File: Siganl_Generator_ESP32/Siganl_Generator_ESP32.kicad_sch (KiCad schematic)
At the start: 25 parts, among them J1 Conn_01x04_Socket, J2 Conn_01x02_Socket, J4 Conn_01x19_Socket, SW1 SW_Push, SW2 SW_Push, SW3 SW_Push, U2 LM393

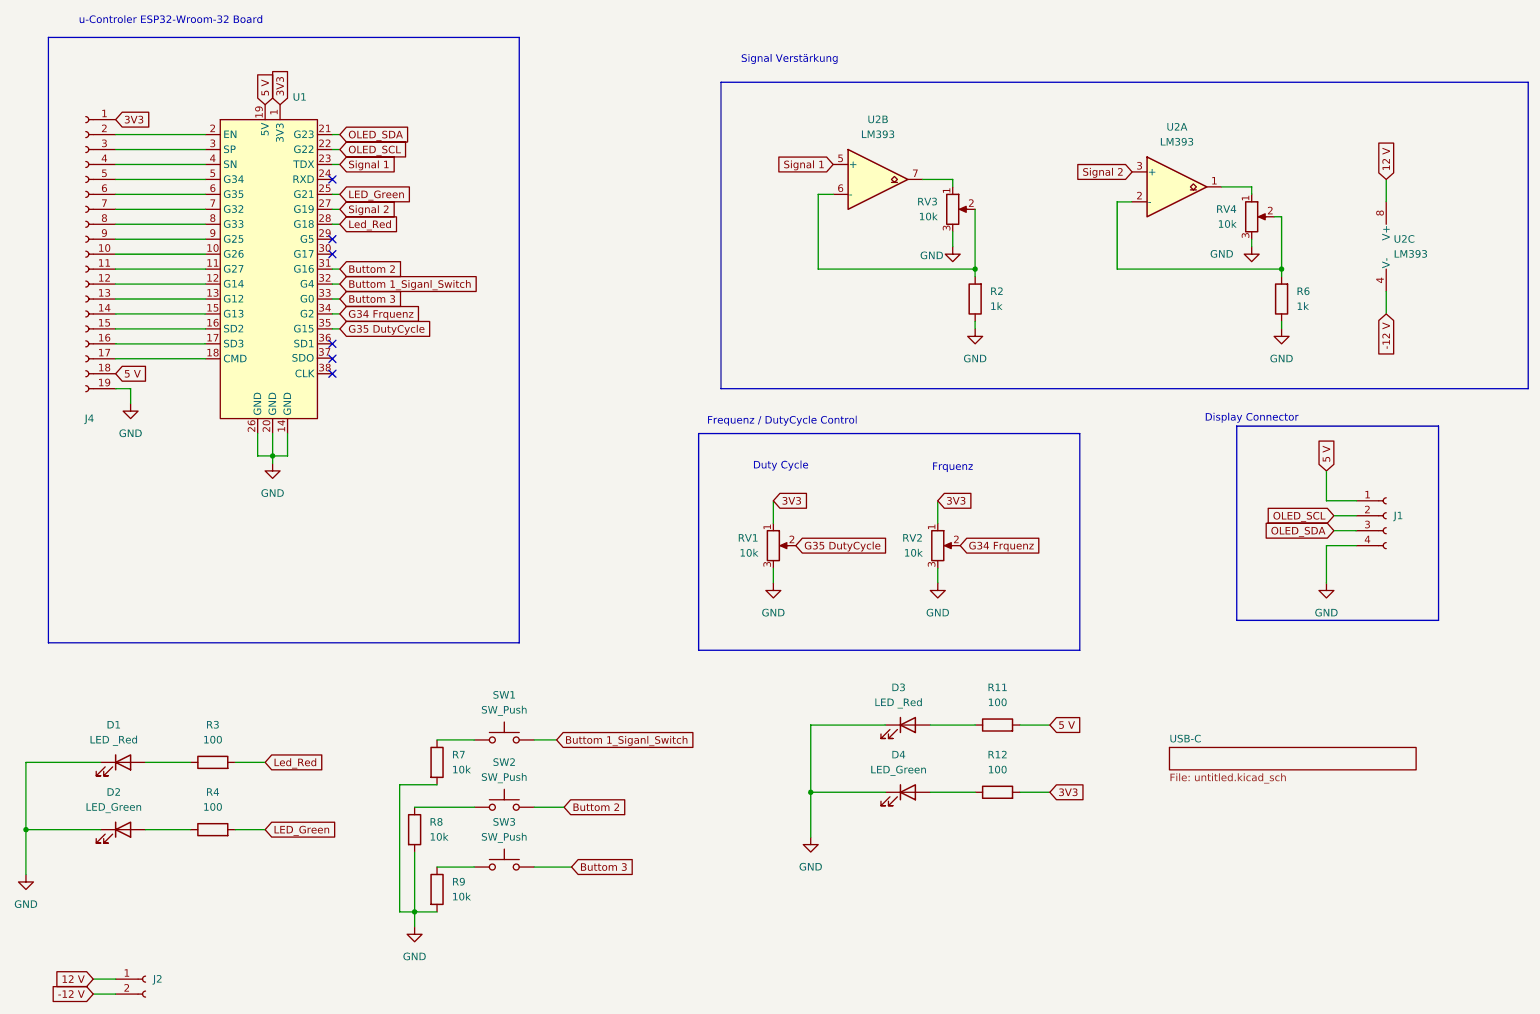
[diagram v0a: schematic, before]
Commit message: klein update
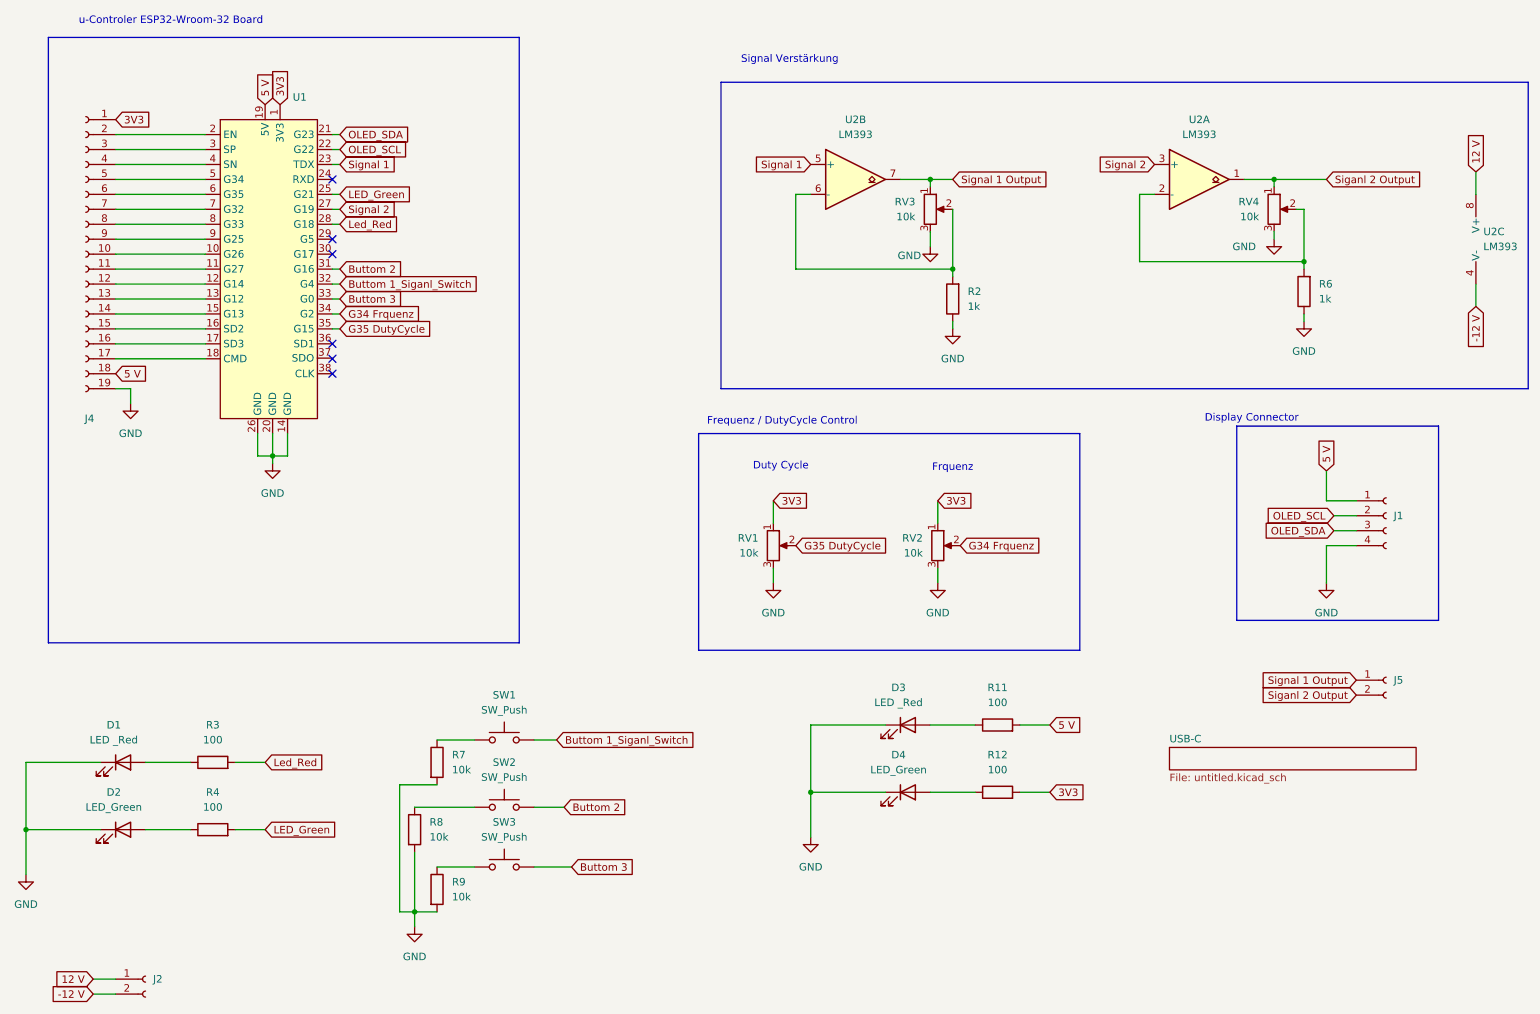
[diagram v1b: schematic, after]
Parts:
- added J5: Conn_01x02_Socket, Connector_PinSocket_2.54mm:PinSocket_1x02_P2.54mm_Vertical, symbol Connector:Conn_01x02_Socket
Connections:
- net Siganl 2 Output: now reaches RV4.1, U2.1
- net Siganl 2 Output: now also J5.2 (Pin_2)
- net Signal 1 Output: now reaches RV3.1, U2.7
- net Signal 1 Output: now also J5.1 (Pin_1)
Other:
- moved on the sheet: R2, R6, RV3, RV4, U2A, U2B, U2C
